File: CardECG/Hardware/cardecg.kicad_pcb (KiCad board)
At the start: 2 copper layers, 63 parts, among them CN1 2TAP, P1 PROG, P2 BATTERY, Q1 NX3008PBKT, Q2 NX3008PBKT, Q3 NX3008PBKT, Q4 NX3008PBKT, Q5 NX3008NBKT, Q6 NX3008NBKT, Q7 NX3008PBKT, Q8 NX3008PBKT, U1 LMV341, U2 LD6815TD/25P, U3 ADuC7061, U4 SSD1306, U5 DNP, U6 DNP, U7 DNP

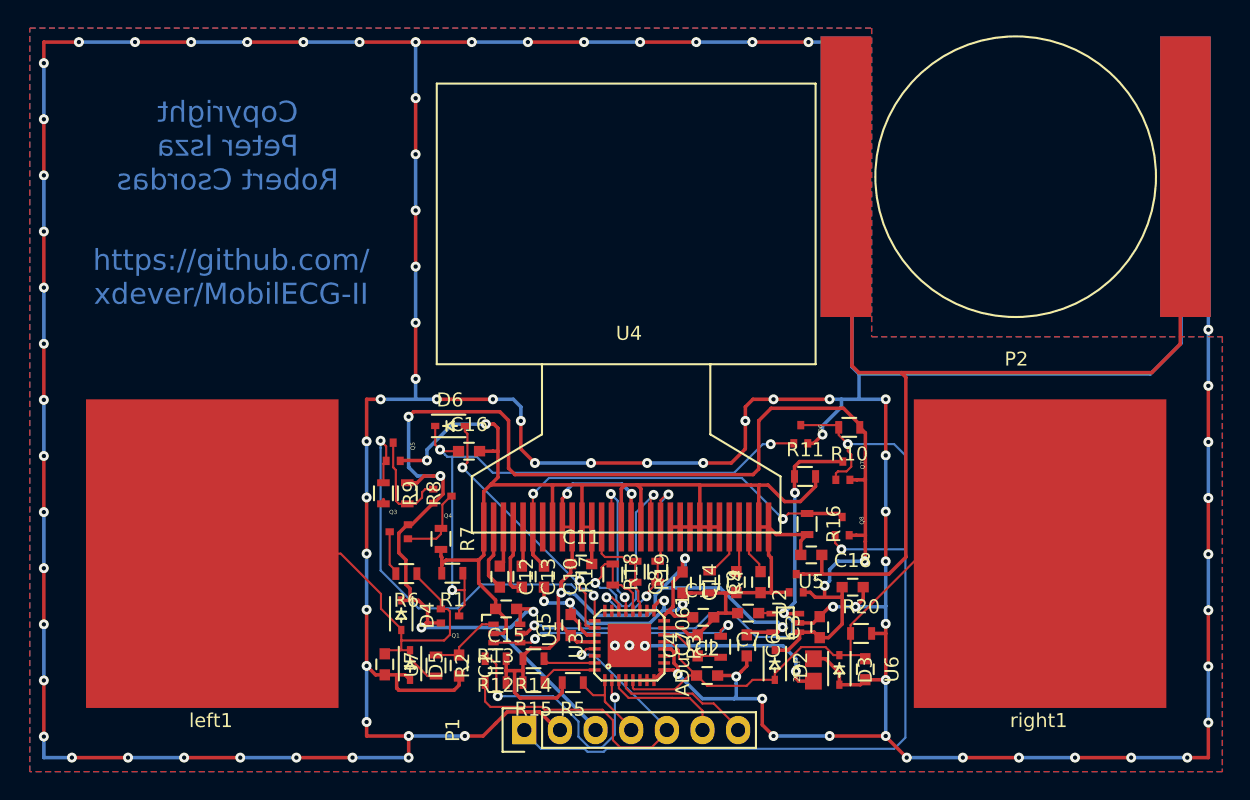
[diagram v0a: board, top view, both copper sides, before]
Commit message: Random modifications.
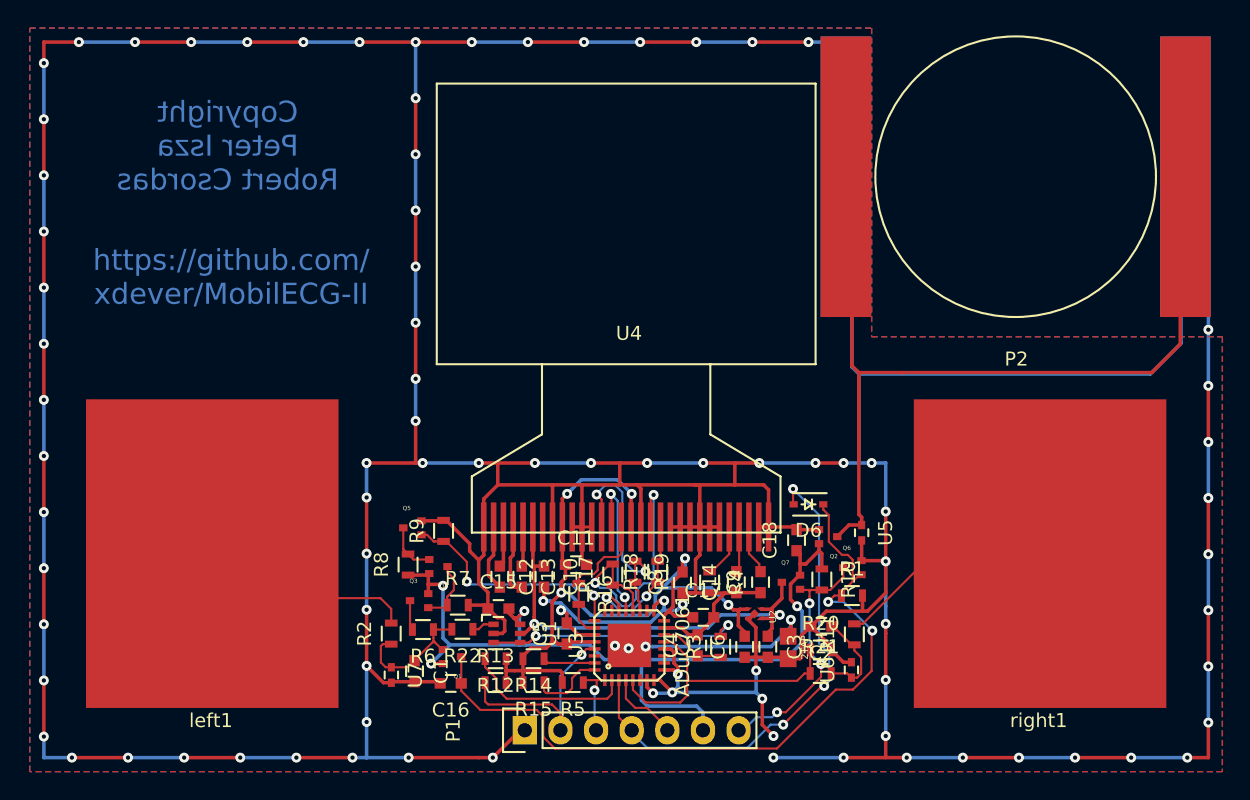
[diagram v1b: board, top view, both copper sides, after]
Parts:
- removed C7: 10nF, Capacitors_SMD:C_0603
- removed D2, D3, D4, D5: D, Diodes_SMD:SOD-323
- removed Q8: NX3008PBKT, mod:SOT416
- added R21: 3.9k, Resistors_SMD:R_0603, F.Cu at (82.4, 70.0)
- added R22: 3.9k, Resistors_SMD:R_0603, F.Cu at (56.8, 66.8)
- C1: value 127pF -> 100pF
- C4: value 100nF -> 8.2nF NP0
- R16: value 47k -> 49
- R3: value 3.9k -> 47k
- R6, R7: value 20M -> 10M
- U2: value LD6815TD/25P -> LD6805K/25; footprint TO_SOT_Packages_SMD:SC-70-5 -> mod:DFN1010C-4
- U5, U6, U7: value DNP -> TPD1E10B06; footprint Capacitors_SMD:C_0603 -> Capacitors_SMD:C_0402
- moved R1 28.5 mm to (84.6, 64.5), turned to 0 degrees
- moved D6 26.2 mm to (81.5, 58.0), turned to 180 degrees
- moved R16 17.0 mm to (65.1, 64.3)
- moved C16 16.6 mm to (56.0, 70.7), turned to 180 degrees
- moved R11 11.8 mm to (84.8, 67.2), turned to 90 degrees
- moved R10 11.0 mm to (82.5, 63.3), turned to 270 degrees
- moved Q6 10.2 mm to (84.6, 62.5), turned to 0 degrees
- moved C2 8.87 mm to (82.4, 66.6), turned to 180 degrees
- moved Q7 8.77 mm to (80.2, 63.5), turned to 0 degrees
- moved Q5 5.59 mm to (53.3, 59.6), turned to 0 degrees
- moved C18 5.22 mm to (80.7, 60.5), turned to 90 degrees
- moved Q3 5.12 mm to (53.8, 64.8)
- moved R8 5.08 mm to (53.0, 62.2), turned to 90 degrees
- moved R9 5.05 mm to (55.5, 59.8), turned to 90 degrees
- moved Q4 5.03 mm to (55.1, 62.4)
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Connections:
- C10 pad 1: OLED_PWR -> VCC
- C15 pad 1: +BATT -> GND
- C15 pad 2: GND -> +BATT
- C3 pad 1: +BATT -> VCC
- C6 pad 1: VDD -> GND
- C6 pad 2: GND -> VDD
- D6 pad 2: POWER_ON -> RX/POWER_ON
- P1 pad 1: ~FORCE_ON -> GND
- P1 pad 2: GND -> ~PROG
- P1 pad 3: +BATT -> ~RESET
- P1 pad 4: ~RESET -> RX/POWER_ON
- P1 pad 5: ~PROG -> TX
- P1 pad 6: RX -> +BATT
- P1 pad 7: TX -> ~FORCE_ON
- Q1 pad 1: Net-(D4-Pad2) -> Net-(C1-Pad1)
- R11 pad 1: VCC -> Net-(C2-Pad1)
- R11 pad 2: GND -> Net-(R11-Pad2)
- R16 pad 1: OLED_PWR -> Net-(R16-Pad1)
- R16 pad 2: GND -> Net-(R16-Pad1)
- R2 pad 2: Net-(D4-Pad2) -> Net-(R2-Pad2)
- R20 pad 1: Net-(C2-Pad1) -> Net-(R20-Pad1)
- R6 pad 1: Net-(D4-Pad2) -> Net-(C1-Pad1)
- U1 pad 1: Net-(C1-Pad1) -> Net-(R22-Pad1)
- U2 pad 1: +BATT -> VDD
- U2 pad 4: Net-(C7-Pad1) -> VCC
- U3 pad 13: Net-(C2-Pad1) -> Net-(R20-Pad1)
- U3 pad 26: POWER_ON -> Net-(R16-Pad1)
- U3 pad 3: RX -> RX/POWER_ON
- U3 pad 5: Net-(C2-Pad1) -> Net-(R20-Pad1)
- U4 pad 10: VDD -> GND
- U4 pad 15: GND -> Net-(R16-Pad1)
- U4 pad 6: OLED_PWR -> VCC
- U7 pad 1: Net-(D4-Pad2) -> Net-(C1-Pad1)
- left1 pad 1: Net-(D4-Pad2) -> Net-(R2-Pad2)
- right1 pad 1: Net-(C2-Pad1) -> Net-(R11-Pad2)
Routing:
- net +BATT: track 114.9 -> 62.1 mm, vias 6 -> 4
- net ~FORCE_ON: track 66.7 -> 18.2 mm, vias 2 -> 3
- net Net-(C2-Pad1): track 52.6 -> 6.77 mm
- net RX/POWER_ON: track 0.00 -> 36.5 mm, vias 0 -> 3
- net Net-(D4-Pad2): track 32.2 -> 0.00 mm
- net OLED_PWR: track 31.2 -> 0.00 mm, vias 2 -> 0
- net GND: track 574.9 -> 549.8 mm, vias 94 -> 89
- net Net-(R20-Pad1): track 0.00 -> 20.6 mm
- net POWER_ON: track 19.0 -> 0.00 mm, vias 2 -> 0
- net Net-(R2-Pad2): track 0.00 -> 15.4 mm
- net Net-(R11-Pad2): track 0.00 -> 15.3 mm
- net PULLUP_OFF: track 31.7 -> 16.8 mm
- net ~PROG: track 26.6 -> 15.4 mm
- net Net-(R16-Pad1): track 0.00 -> 10.6 mm
- net Net-(P2-Pad1): track 77.2 -> 67.2 mm
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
